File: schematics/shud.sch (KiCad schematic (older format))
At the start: 11 parts, among them P1 JTAG, U1 STM32F303_K8T6, U2 APE8865N-33-HF-3

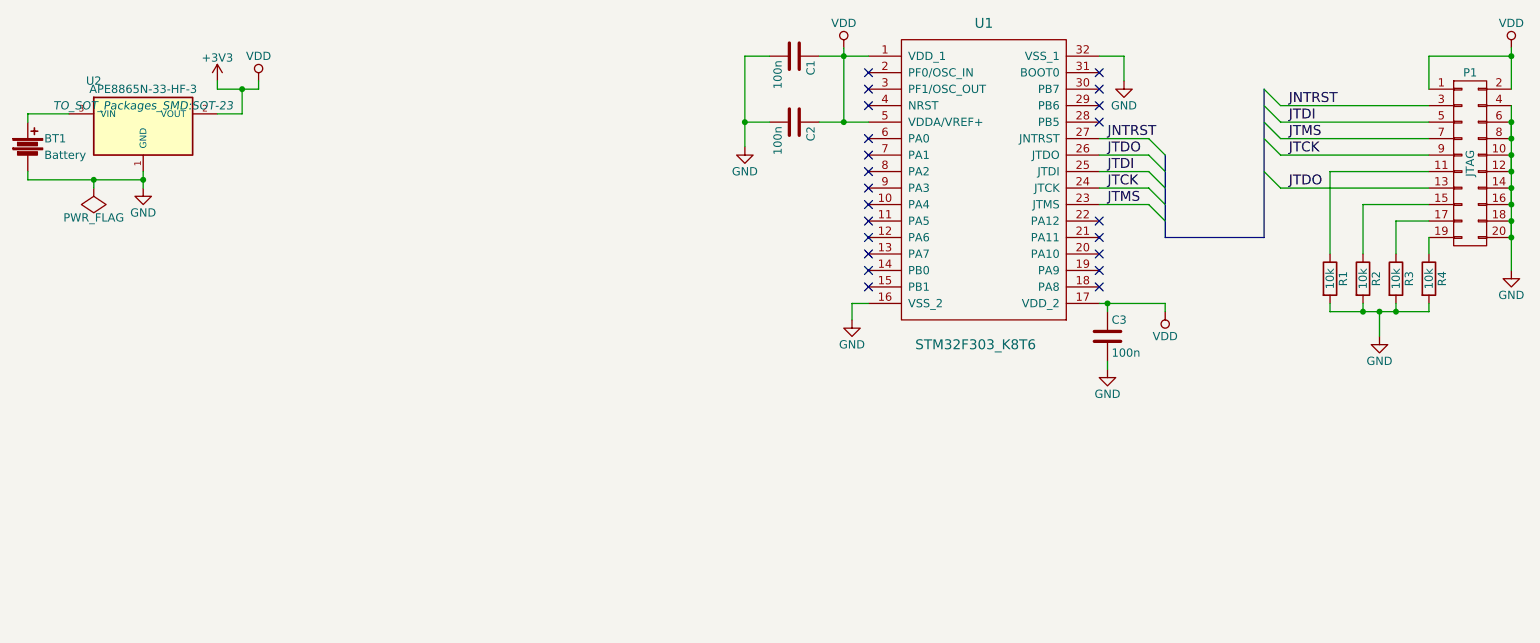
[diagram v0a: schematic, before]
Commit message: finish pcb
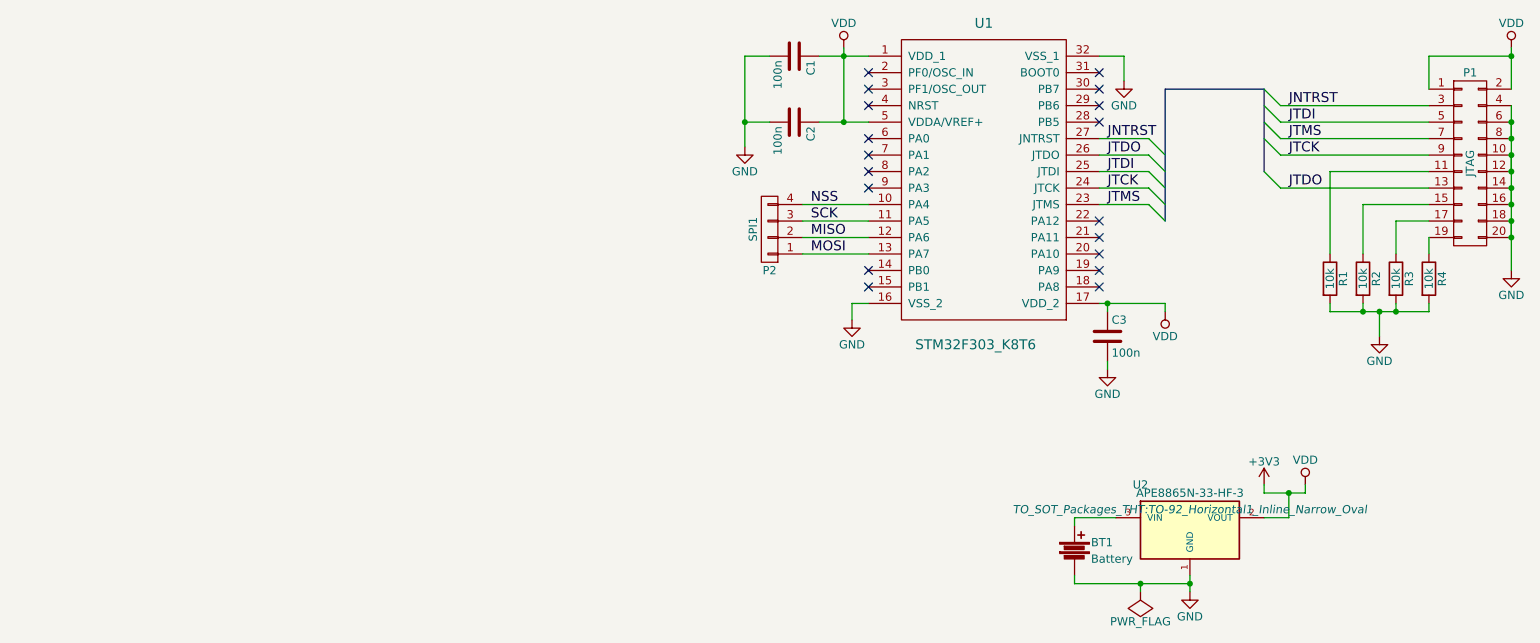
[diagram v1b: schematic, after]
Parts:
- added P2: SPI1, Pin_Headers:Pin_Header_Straight_1x04, symbol CONN_01X04
- BT1: footprint Pin_Headers:Pin_Header_Straight_1x02 -> Terminal_Blocks:TerminalBlock_Pheonix_MKDS1.5-2pol
- R1, R2, R3, R4: footprint Resistors_ThroughHole:Resistor_Cement_Horizontal_Meggitt-SBC-2 -> Resistors_ThroughHole:Resistor_Horizontal_RM10mm
- U2: footprint TO_SOT_Packages_SMD:SOT-23 -> TO_SOT_Packages_THT:TO-92_Horizontal1_Inline_Narrow_Oval
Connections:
- net NSS: now reaches U1.10 (PA4)
- net NSS: now also P2.4 (P4)
- net SCK: now reaches U1.11 (PA5)
- net SCK: now also P2.3 (P3)
- net MISO: now reaches U1.12 (PA6)
- net MISO: now also P2.2 (P2)
- net MOSI: now reaches U1.13 (PA7)
- net MOSI: now also P2.1 (P1)
- no-connect marks 22 -> 18
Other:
- moved on the sheet: BT1, U2
